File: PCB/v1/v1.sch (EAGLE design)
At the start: 64 parts, among them U2 AT24C512C-SHD-B

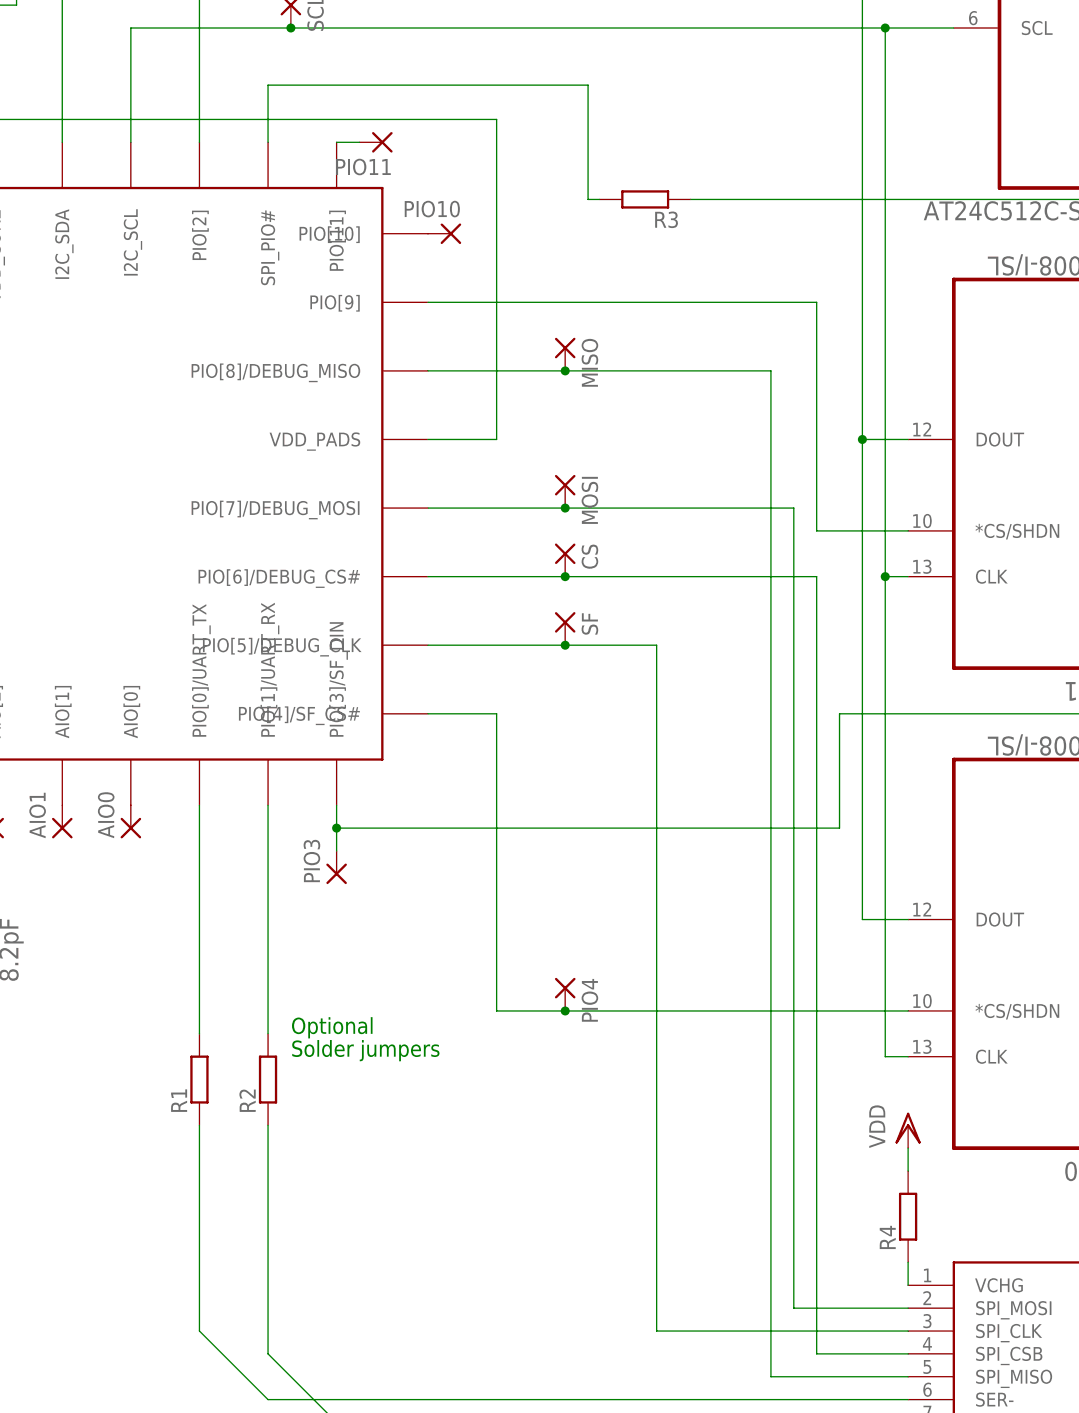
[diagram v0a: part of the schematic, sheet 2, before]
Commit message: push to work from main pc
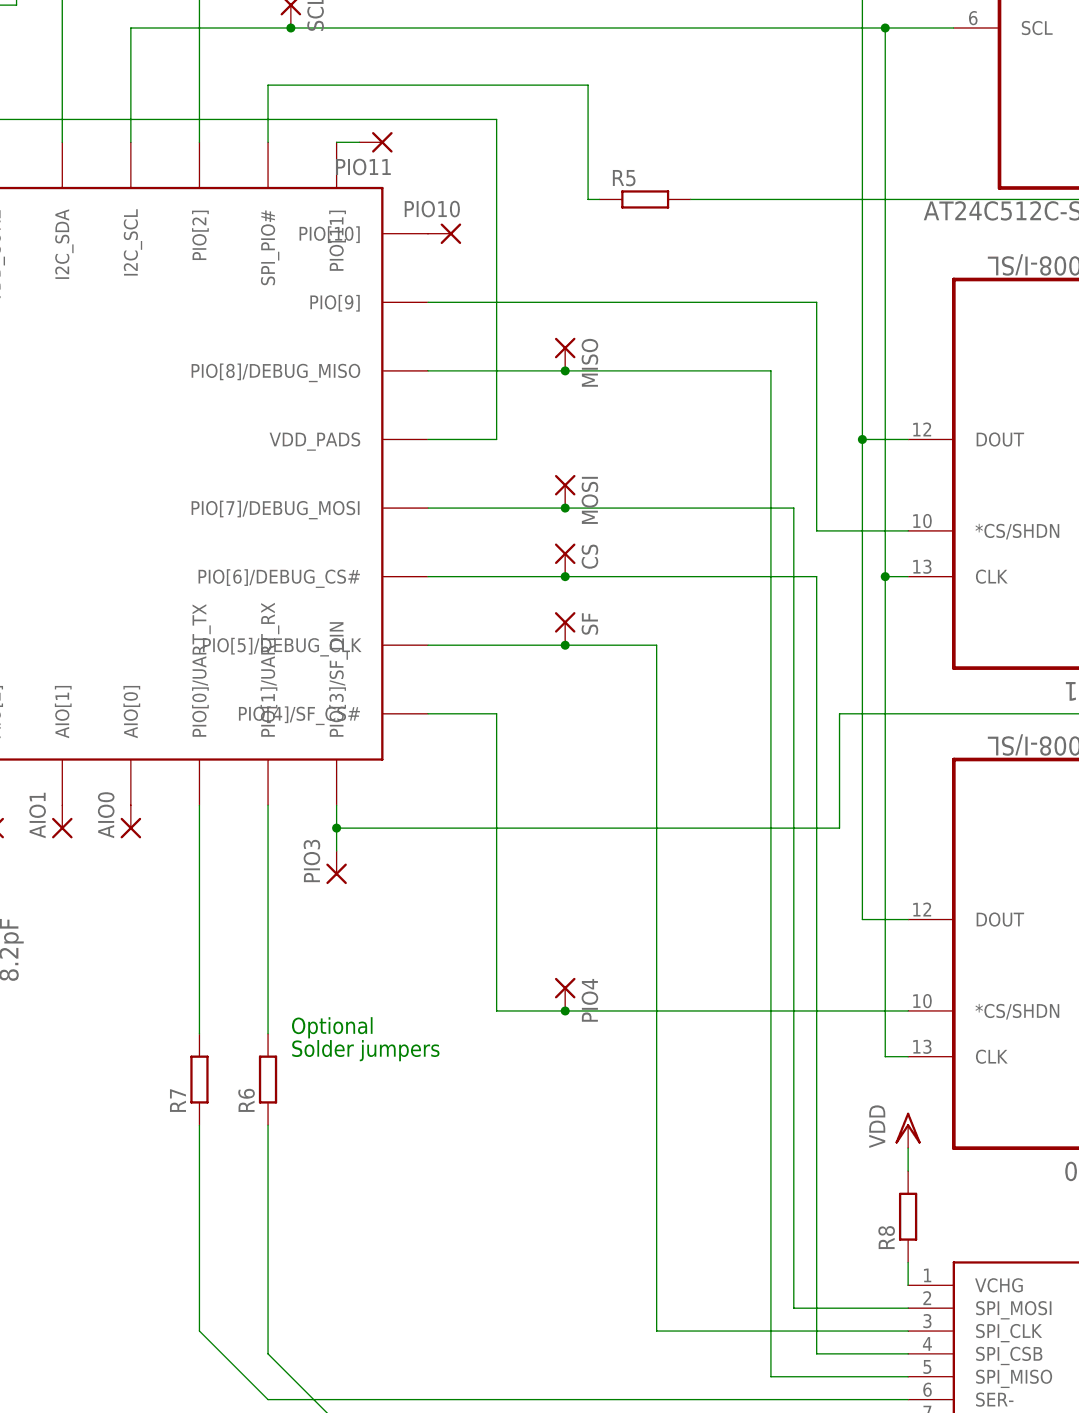
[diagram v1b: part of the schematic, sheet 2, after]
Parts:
- removed R1, R2, R3, R4: (no value), resistor-shunt:BVS
- added R5, R6, R7, R8: (no value), eagle-ltspice:RR1206
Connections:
- net N$20: now also R7.1; no longer R1.2
- net N$36: now also R6.1; no longer R2.2
- net N$37: now also R7.2; no longer R1.1
- net N$38: now also R6.2; no longer R2.1
- net N$40: now also R8.1; no longer R4.2
- net N$45: now also R5.1; no longer R3.1
- net VDD: now also R5.2, R8.2; no longer R3.2, R4.1

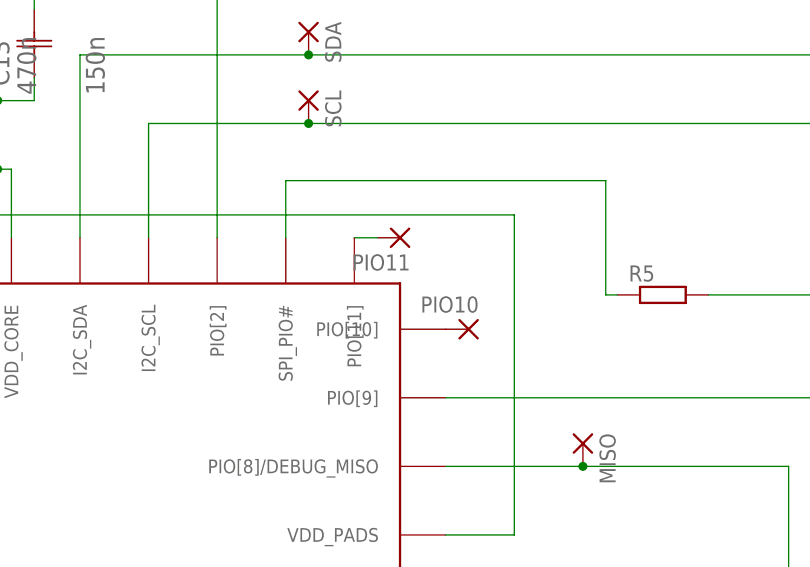
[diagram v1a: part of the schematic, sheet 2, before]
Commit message: takes its time
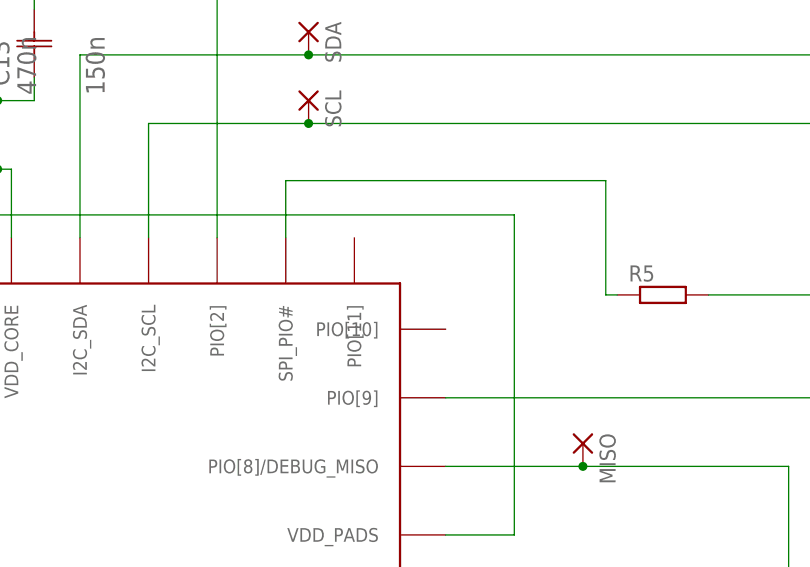
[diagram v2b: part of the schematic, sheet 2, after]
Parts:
- removed PIO10, PIO11: (no value), wirepad:1,6/0,8
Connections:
- removed net N$42: PIO10.P, U$1.PIO[10]
- removed net N$47: PIO11.P, U$1.PIO[11]
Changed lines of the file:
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@@
 <part name="AIO0" library="wirepad" deviceset="1,6/0,8" device=""/>
 <part name="PIO3" library="wirepad" deviceset="1,6/0,8" device=""/>
-<part name="PIO10" library="wirepad" deviceset="1,6/0,8" device=""/>
-<part name="PIO11" library="wirepad" deviceset="1,6/0,8" device=""/>
 <part name="C1" library="AVX_By_element14_Batch_1" deviceset="UQCL2A100JAT2A/500" device="" value="1u"/>
 <part name="VPLUS" library="solpad" deviceset="LSP10" device="" value="Vrail"/>
@@
 <instance part="AIO0" gate="P" x="-55.88" y="15.24" rot="R90"/>
 <instance part="PIO3" gate="P" x="-33.02" y="10.16" rot="R90"/>
-<instance part="PIO10" gate="P" x="-20.32" y="81.28" rot="MR0"/>
-<instance part="PIO11" gate="P" x="-27.94" y="91.44" rot="R180"/>
 <instance part="C1" gate="A" x="73.152" y="108.204" rot="R90"/>
 <instance part="VPLUS" gate="1" x="-157.48" y="114.3" rot="R270"/>
@@
 </segment>
 </net>
-<net name="N$47" class="0">
-<segment>
-<pinref part="PIO11" gate="P" pin="P"/>
-<wire x1="-33.02" y1="91.44" x2="-30.48" y2="91.44" width="0.1524" layer="91"/>
-<pinref part="U$1" gate="G$1" pin="PIO[11]"/>
-</segment>
-</net>
 <net name="N$48" class="0">
 <segment>
@@
 </segment>
 </net>
-<net name="N$42" class="0">
-<segment>
-<pinref part="PIO10" gate="P" pin="P"/>
-<pinref part="U$1" gate="G$1" pin="PIO[10]"/>
-</segment>
-</net>

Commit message: getting there
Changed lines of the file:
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@@
 <wire x1="-129.54" y1="101.6" x2="-137.16" y2="101.6" width="0.1524" layer="91"/>
 <junction x="-137.16" y="101.6"/>
-<wire x1="-137.16" y1="101.6" x2="-144.78" y2="101.6" width="0.1524" layer="91"/>
 <pinref part="C19" gate="A" pin="C1"/>
 <wire x1="-154.94" y1="101.6" x2="-144.78" y2="101.6" width="0.1524" layer="91"/>
@@
 <junction x="-157.48" y="71.12"/>
 <pinref part="U$6" gate="G$1" pin="NEG"/>
+<wire x1="-144.78" y1="101.6" x2="-137.16" y2="101.6" width="0.1524" layer="91"/>
 </segment>
 <segment>

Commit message: quickly added antenna
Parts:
- added U$7: ANTENNA_1LEFT, ant-planar-1:ANTENNA_1LEFT
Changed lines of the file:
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@@
 <part name="R7" library="eagle-ltspice" deviceset="R" device="R1206"/>
 <part name="R8" library="eagle-ltspice" deviceset="R" device="R1206"/>
+<part name="U$7" library="ant-planar-1" deviceset="ANTENNA_1" device="LEFT"/>
 </parts>
 <sheets>
-<sheet>
-<plain>
-</plain>
-<instances>
-</instances>
-<busses>
-</busses>
-<nets>
-</nets>
-</sheet>
 <sheet>
 <plain>
@@
 <instance part="GND7" gate="1" x="-129.54" y="15.24"/>
 <instance part="C14" gate="A" x="-101.6" y="10.16" rot="R90"/>
-<instance part="GND9" gate="1" x="-165.1" y="27.94"/>
+<instance part="GND9" gate="1" x="-152.4" y="25.4"/>
 <instance part="C16" gate="A" x="-137.16" y="109.22" rot="R270"/>
 <instance part="C17" gate="A" x="-129.54" y="109.22" rot="R270"/>
@@
 <instance part="R7" gate="G$1" x="-48.26" y="-12.7" rot="R90"/>
 <instance part="R8" gate="G$1" x="30.48" y="-27.94" rot="R90"/>
+<instance part="U$7" gate="G$1" x="-157.48" y="45.72"/>
 </instances>
 <busses>
@@
 </segment>
 <segment>
+<pinref part="C10" gate="A" pin="C1"/>
+<pinref part="C11" gate="A" pin="C1"/>
+<wire x1="-137.16" y1="20.32" x2="-129.54" y2="20.32" width="0.1524" layer="91"/>
+<pinref part="GND7" gate="1" pin="GND"/>
+<wire x1="-129.54" y1="17.78" x2="-129.54" y2="20.32" width="0.1524" layer="91"/>
+<junction x="-129.54" y="20.32"/>
+<wire x1="-129.54" y1="20.32" x2="-121.92" y2="20.32" width="0.1524" layer="91"/>
+</segment>
+<segment>
 <pinref part="GND9" gate="1" pin="GND"/>
-<wire x1="-165.1" y1="35.56" x2="-165.1" y2="30.48" width="0.1524" layer="91"/>
+<wire x1="-152.4" y1="33.02" x2="-152.4" y2="27.94" width="0.1524" layer="91"/>
 </segment>
 <segment>
@@
 <wire x1="-83.82" y1="119.38" x2="-76.2" y2="119.38" width="0.1524" layer="91"/>
 <junction x="-76.2" y="119.38"/>
-</segment>
-<segment>
-<pinref part="C11" gate="A" pin="C1"/>
-<pinref part="C10" gate="A" pin="C1"/>
-<wire x1="-137.16" y1="20.32" x2="-129.54" y2="20.32" width="0.1524" layer="91"/>
-<pinref part="GND7" gate="1" pin="GND"/>
-<wire x1="-129.54" y1="20.32" x2="-121.92" y2="20.32" width="0.1524" layer="91"/>
-<wire x1="-129.54" y1="17.78" x2="-129.54" y2="20.32" width="0.1524" layer="91"/>
-<junction x="-129.54" y="20.32"/>
 </segment>
 </net>
@@
 <wire x1="-96.52" y1="35.56" x2="-109.22" y2="35.56" width="0.1524" layer="91"/>
 <pinref part="U$1" gate="G$1" pin="RF"/>
-</segment>
-</net>
+<wire x1="-109.22" y1="35.56" x2="-152.4" y2="35.56" width="0.1524" layer="91"/>
+<junction x="-109.22" y="35.56"/>
+</segment>
+</net>

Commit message: latest
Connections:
- net GND: now also U$5.NEG; no longer U$6.NEG
- net N$34: now also U$6.POS; no longer U$5.POS
- net N$48: now also U$5.POS, U$6.NEG; no longer U$5.NEG, U$6.POS
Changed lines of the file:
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@@
 <part name="U$2" library="MINI_SMT_8_PIN_CONNECTOR" deviceset="8PIN_SMT_CONNECTOR" device=""/>
 <part name="U$4" library="SSP-T7-F" deviceset="SSP-T7-F" device=""/>
-<part name="U$5" library="BATTERY_2996" deviceset="BATTERY_2996" device=""/>
-<part name="U$6" library="BATTERY_2996" deviceset="BATTERY_2996" device=""/>
 <part name="R5" library="eagle-ltspice" deviceset="R" device="R1206"/>
 <part name="R6" library="eagle-ltspice" deviceset="R" device="R1206"/>
@@
 <part name="R8" library="eagle-ltspice" deviceset="R" device="R1206"/>
 <part name="U$7" library="ant-planar-1" deviceset="ANTENNA_1" device="LEFT"/>
+<part name="U$5" library="BATTERY_2996" deviceset="BATTERY_2996" device=""/>
+<part name="U$6" library="BATTERY_2996" deviceset="BATTERY_2996" device=""/>
 </parts>
 <sheets>
@@
 <instance part="U$2" gate="G$1" x="43.18" y="-48.26"/>
 <instance part="U$4" gate="G$1" x="-109.22" y="69.85" rot="R270"/>
-<instance part="U$5" gate="G$1" x="-172.72" y="101.6"/>
-<instance part="U$6" gate="G$1" x="-172.72" y="78.74"/>
 <instance part="R5" gate="G$1" x="1.27" y="85.09"/>
 <instance part="R6" gate="G$1" x="-40.64" y="-12.7" rot="R90"/>
@@
 <instance part="R8" gate="G$1" x="30.48" y="-27.94" rot="R90"/>
 <instance part="U$7" gate="G$1" x="-157.48" y="45.72"/>
+<instance part="U$5" gate="G$1" x="-172.72" y="78.74"/>
+<instance part="U$6" gate="G$1" x="-172.72" y="101.6"/>
 </instances>
 <busses>
@@
 <pinref part="VGND" gate="1" pin="MP"/>
 <junction x="-157.48" y="71.12"/>
-<pinref part="U$6" gate="G$1" pin="NEG"/>
 <wire x1="-144.78" y1="101.6" x2="-137.16" y2="101.6" width="0.1524" layer="91"/>
+<pinref part="U$5" gate="G$1" pin="NEG"/>
 </segment>
 <segment>
@@
 <pinref part="U$1" gate="G$1" pin="VDD_PADS"/>
 <pinref part="U$1" gate="G$1" pin="VDD_BAT_SMPS"/>
-<pinref part="U$5" gate="G$1" pin="POS"/>
+<pinref part="U$6" gate="G$1" pin="POS"/>
 </segment>
 </net>
@@
 <segment>
 <wire x1="-162.56" y1="93.98" x2="-162.56" y2="86.36" width="0.1524" layer="91"/>
-<pinref part="U$5" gate="G$1" pin="NEG"/>
-<pinref part="U$6" gate="G$1" pin="POS"/>
-</segment>
-</net>
+<pinref part="U$5" gate="G$1" pin="POS"/>
+<pinref part="U$6" gate="G$1" pin="NEG"/>
+</segment>
+</net>
